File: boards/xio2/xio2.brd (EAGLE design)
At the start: 170 x 100 mm, 337 parts, among them J1 12401598E4#2A, Q1 BSS138, Q2 BSS138, Q3 BC817-16LT3G, Q4 BC817-16LT3G, Y2 FA-238 25.0000MB-K3

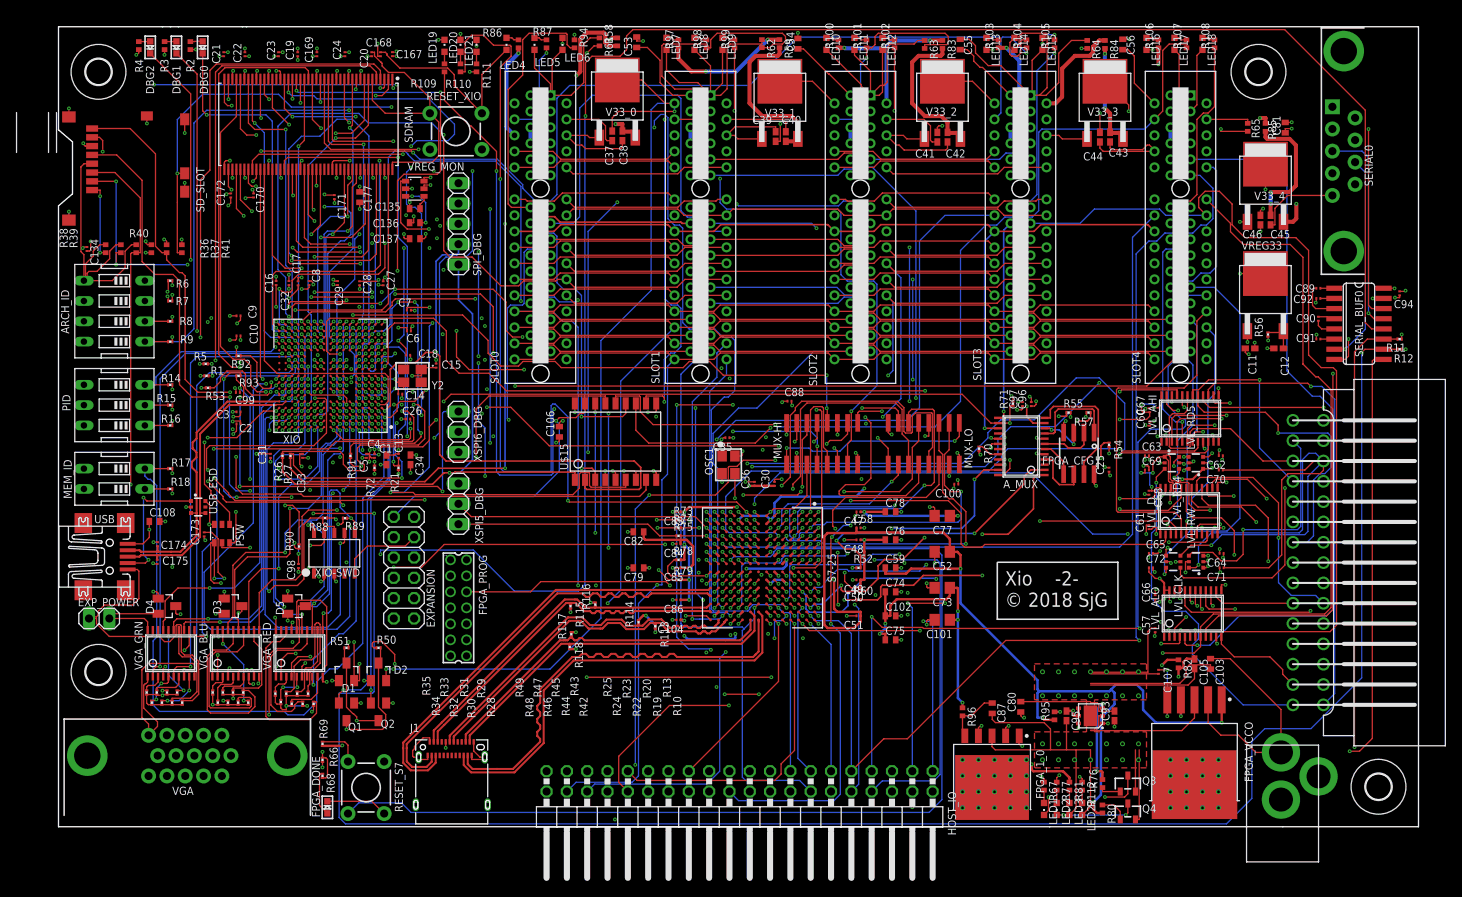
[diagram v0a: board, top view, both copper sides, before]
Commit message: Simple changes from design reviews completed.
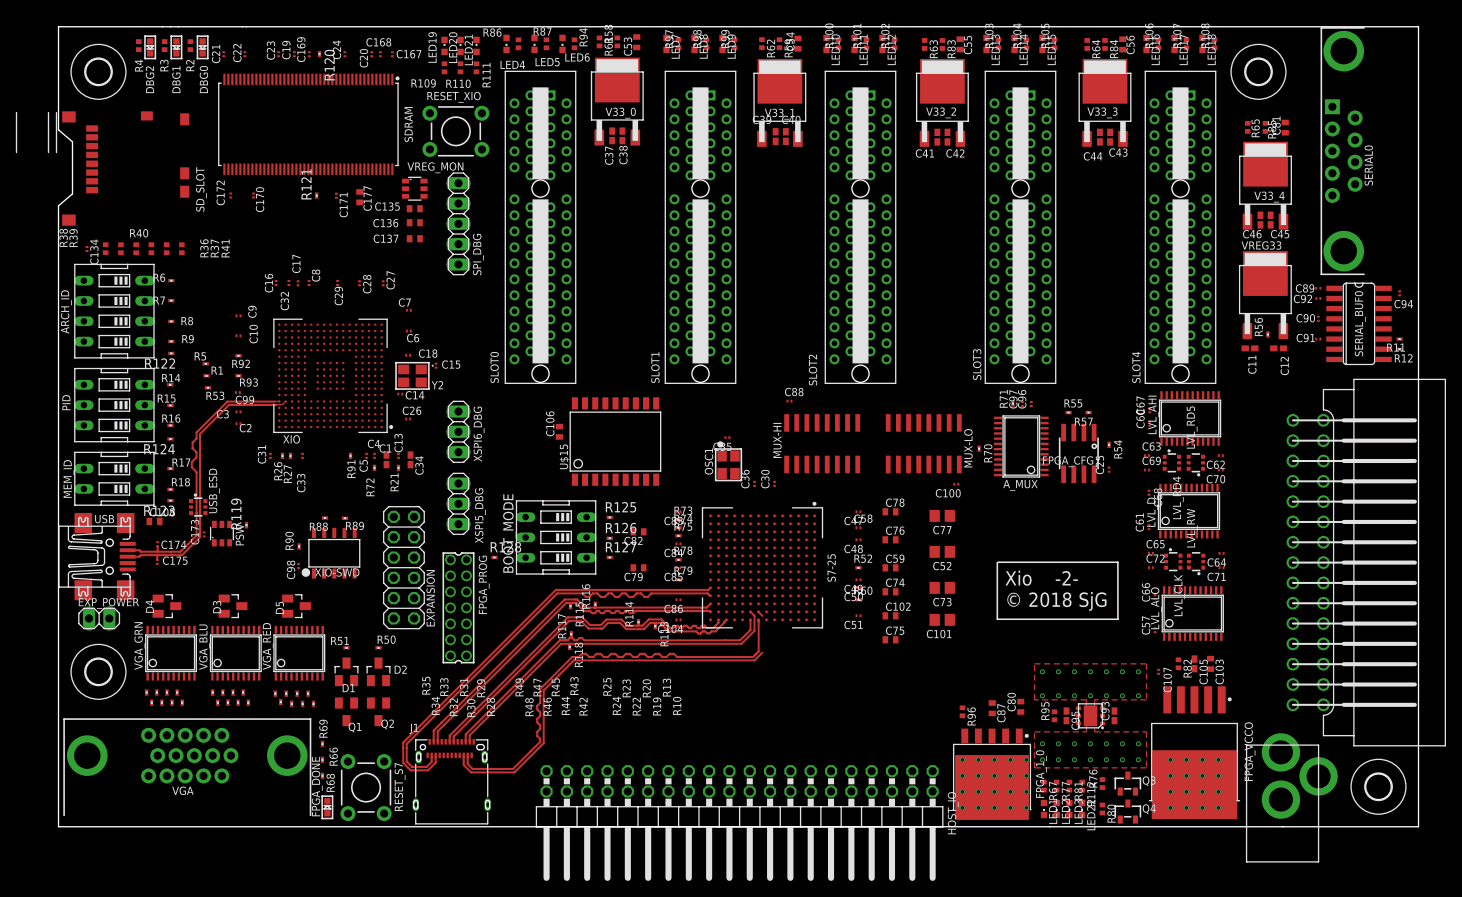
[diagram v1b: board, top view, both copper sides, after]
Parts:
- added BOOT_MODE: 209-3MS, special:EDG-03
- added R119: 100K, rcl:R0201
- added R120, R121: 10K, rcl:R0201
- added R122, R123, R124, R128: 1K, rcl:R0201
- added R125, R126, R127: 47K, rcl:R0201
- C173: value 0.1uF -> 1uF
- moved C169 0.95 mm to (31.4, 97.2)
- moved C19 0.42 mm to (29.5, 97.2)
- moved C171 0.31 mm to (34.7, 79.5)
- moved R7 0.14 mm to (14.1, 66.4), turned to 0 degrees
- moved R9 0.13 mm to (14.1, 61.3)
- moved R8 0.13 mm to (14.1, 63.8)
- moved R6 0.13 mm to (14.1, 68.9), turned to 0 degrees
- moved R18 0.07 mm to (14.0, 42.8)
- moved R15 0.05 mm to (14.0, 53.3)
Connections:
- net SPI_IRQ renamed !SPI_IRQ!
- new net BOOT_M0: BOOT_MODE.1, R127.1, S7-25.M7
- new net BOOT_M1: BOOT_MODE.2, R126.1, S7-25.M8
- new net BOOT_M2: BOOT_MODE.3, R125.1, S7-25.M9
- new net N$11: ARCH_ID.5, ARCH_ID.6, ARCH_ID.7, ARCH_ID.8, R122.2
- new net N$2: R121.2, SDRAM.67
- new net N$48: MEM_ID.3, MEM_ID.4, R123.2
- new net N$49: PID.4, PID.5, PID.6, R124.2
- new net N$50: BOOT_MODE.4, BOOT_MODE.5, BOOT_MODE.6, R128.2
- new net N$7: R120.1, SDRAM.20
- net +3V3: now also R121.1, R122.1, R123.1, R124.1, R128.1; no longer ARCH_ID.5, ARCH_ID.6, ARCH_ID.7, ARCH_ID.8, LVL_RD4.5, LVL_RD5.5, MEM_ID.3, MEM_ID.4, MUX-HI.16, MUX-LO.16, PID.4, PID.5, PID.6, S7-25.M7, SDRAM.67
- net +5V: now also LVL_RD4.5, LVL_RD5.5, R119.1
- net GND: now also R120.2, R125.2, R126.2, R127.2; no longer S7-25.M8, S7-25.M9, SDRAM.20
- net N$65: now also R119.2
- net VCCO: now also MUX-HI.16, MUX-LO.16
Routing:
- net GND: track 794.0 -> 0.00 mm, vias 347 -> 64
- net +5V: track 594.2 -> 0.00 mm, vias 47 -> 0
- net HOST_A3: track 362.8 -> 0.00 mm, vias 6 -> 0
- net HOST_A7: track 329.8 -> 0.00 mm, vias 6 -> 0
- net HOST_A6: track 316.2 -> 0.00 mm, vias 6 -> 0
- net HOST_A5: track 311.9 -> 0.00 mm, vias 7 -> 0
- net HOST_A2: track 307.1 -> 0.00 mm, vias 4 -> 0
- net HOST_A0: track 301.8 -> 0.00 mm, vias 7 -> 0
- net HOST_A10: track 295.2 -> 0.00 mm, vias 10 -> 0
- net HOST_A4: track 284.1 -> 0.00 mm, vias 6 -> 0
- net MCU_TX: track 282.2 -> 0.00 mm, vias 3 -> 0
- net HOST_A14: track 270.9 -> 0.00 mm, vias 8 -> 0
- net HOST_A8: track 266.2 -> 0.00 mm, vias 7 -> 0
- net HOST_A12: track 262.5 -> 0.00 mm, vias 7 -> 0
- net VCCO: track 261.9 -> 0.00 mm, vias 28 -> 0
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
